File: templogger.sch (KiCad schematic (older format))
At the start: 20 parts, among them J1 USB_A, J2 Conn_01x03, U1 MCP2221, U2 ATtiny3216-S, U3 LM35-LP, U4 SC39_11_RT, U5 SC39_11_RT, U6 SC_39_11_RT, U7 SC_39_11_RT

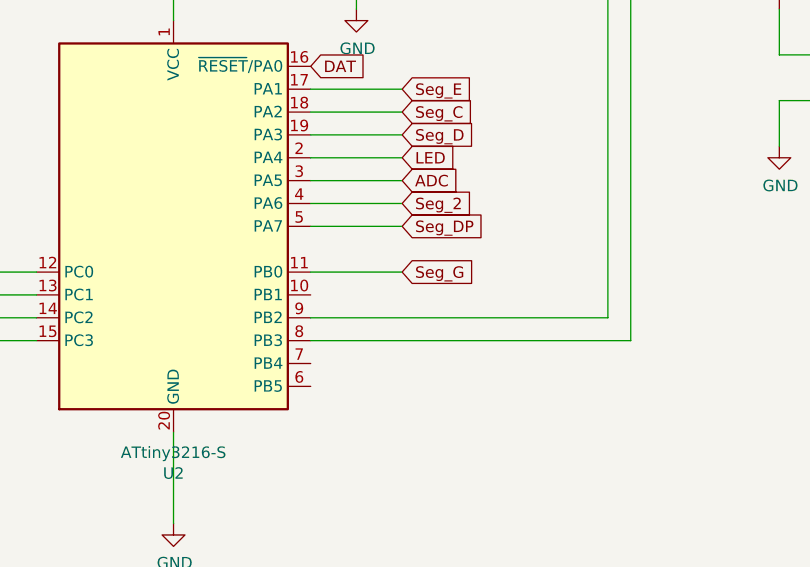
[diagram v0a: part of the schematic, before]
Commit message: First PCB Layout
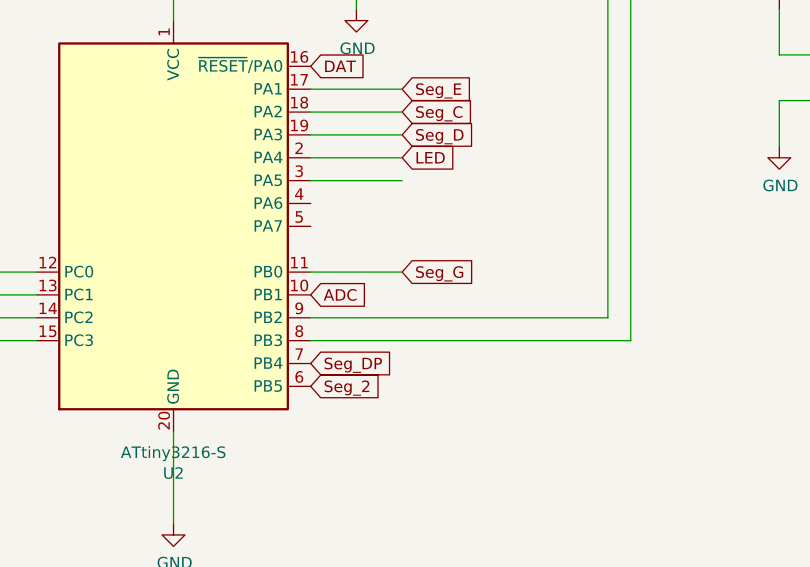
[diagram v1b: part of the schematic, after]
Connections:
- net ADC: now also U2.10 (PB1); no longer U2.3 (PA5)
- net Seg_2: now also U2.6 (PB5); no longer U2.4 (PA6)
- net Seg_DP: now also U2.7 (PB4); no longer U2.5 (PA7)
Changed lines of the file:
@@
 Wire Wire Line
 	6100 5100 6500 5100
-Wire Wire Line
-	6100 5200 6500 5200
-Wire Wire Line
-	6100 5300 6500 5300
-Text GLabel 6500 5300 2    50   Input ~ 0
+Text GLabel 6100 5900 2    50   Input ~ 0
 Seg_DP
-Text GLabel 6500 5200 2    50   Input ~ 0
+Text GLabel 6100 6000 2    50   Input ~ 0
 Seg_2
-Text GLabel 6500 5100 2    50   Input ~ 0
+Text GLabel 6100 5600 2    50   Input ~ 0
 ADC
 Text GLabel 6500 5000 2    50   Input ~ 0
@@
 Seg_F
 $Comp
-L power:GND #PWR?
+L power:GND #PWR0118
 U 1 1 5EC8A53C
 P 4500 3100
-F 0 "#PWR?" H 4500 2850 50  0001 C CNN
+F 0 "#PWR0118" H 4500 2850 50  0001 C CNN
 F 1 "GND" H 4505 2927 50  0000 C CNN
 F 2 "" H 4500 3100 50  0001 C CNN
